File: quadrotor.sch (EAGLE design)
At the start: 10 parts, among them X1 16MHZ

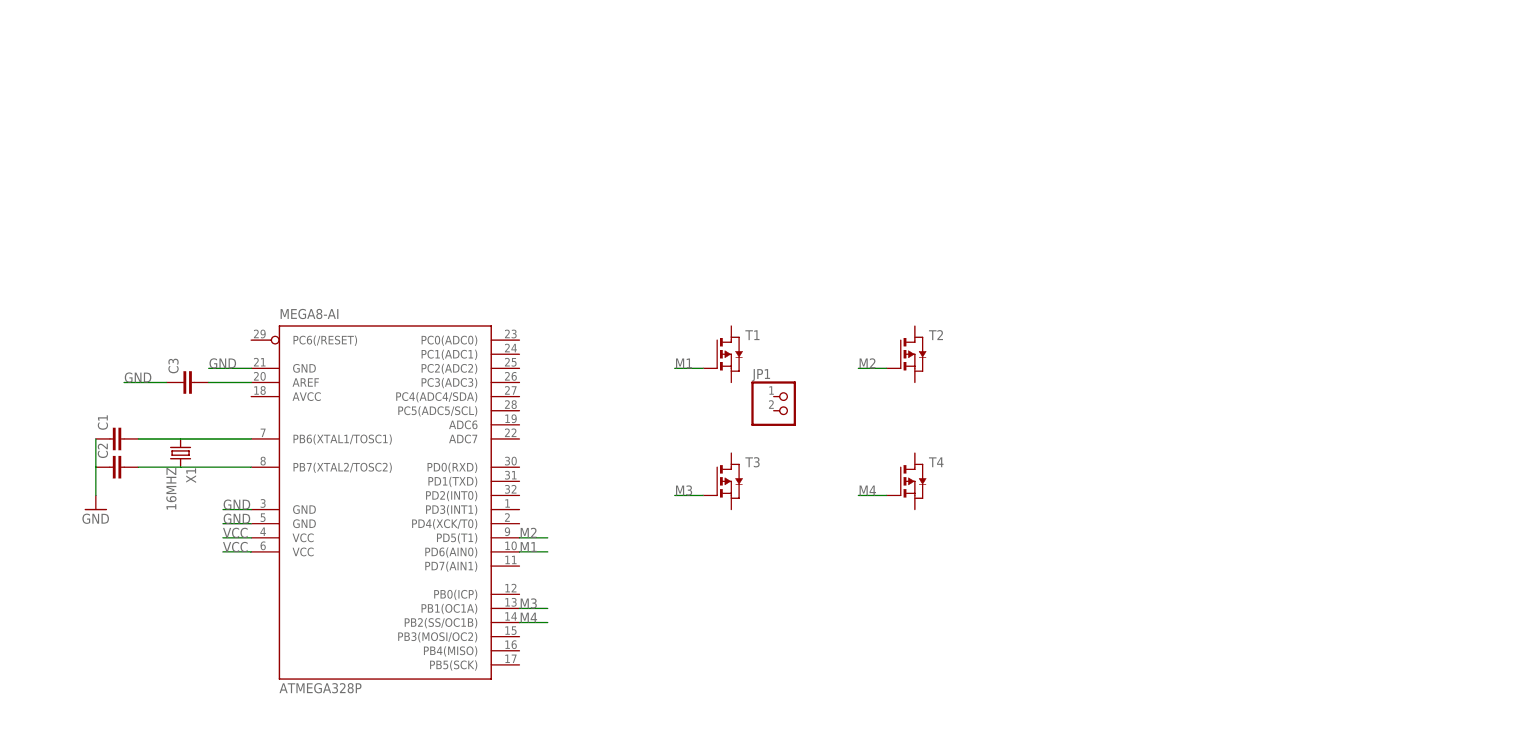
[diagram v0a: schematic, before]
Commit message: done bluetooth protocal
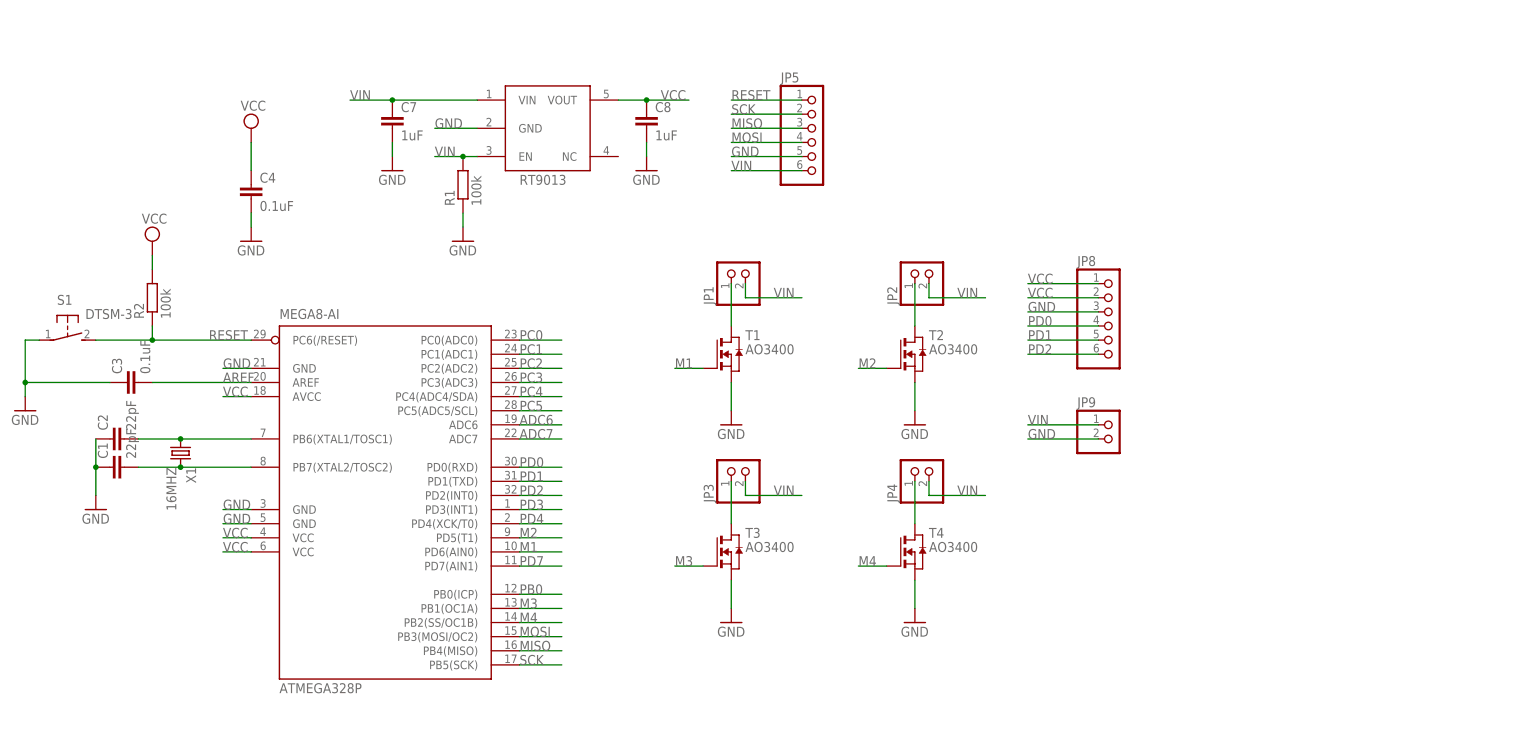
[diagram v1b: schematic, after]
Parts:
- added C4: 0.1uF, eagle-ltspice:CC0603
- added C7, C8: 1uF, eagle-ltspice:CC0603
- added JP2, JP3, JP4: (no value), pinhead:PINHD-1X2
- added JP5: (no value), pinhead:PINHD-1X6/90
- added JP8: (no value), pinhead:PINHD-1X6
- added JP9: (no value), pinhead:PINHD-1X2/90
- added R1, R2: 100k, eagle-ltspice:RR0603
- added S1: DTSM-3, switch-tact:DTSM-3
- added U$1: RT9013, quadrotor:RT9013
- C1, C2: value (none) -> 22pF
- C3: value (none) -> 0.1uF
- T1, T2, T3, T4: value (none) -> AO3400; device zetex:PMOSSOT23 -> zetex:NMOSSOT23
- X1: device IQD-Frequency-Products:CRYSTALS-NOGND-HC49 -> IQD-Frequency-Products:CRYSTALS-NOGND-12SMX-A
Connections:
- net N$3 renamed AREF
- new net ADC6: ATMEGA328P.ADC6
- new net ADC7: ATMEGA328P.ADC7
- new net MISO: ATMEGA328P.PB4(MISO), JP5.3
- new net MOSI: ATMEGA328P.PB3(MOSI/OC2), JP5.4
- new net N$10: JP3.1, T3.D
- new net N$4: JP1.1, T1.D
- new net N$6: JP2.1, T2.D
- new net N$9: JP4.1, T4.D
- new net PB0: ATMEGA328P.PB0(ICP)
- new net PC0: ATMEGA328P.PC0(ADC0)
- new net PC1: ATMEGA328P.PC1(ADC1)
- new net PC2: ATMEGA328P.PC2(ADC2)
- new net PC3: ATMEGA328P.PC3(ADC3)
- new net PC4: ATMEGA328P.PC4(ADC4/SDA)
- new net PC5: ATMEGA328P.PC5(ADC5/SCL)
- new net PD0: ATMEGA328P.PD0(RXD), JP8.4
- new net PD1: ATMEGA328P.PD1(TXD), JP8.5
- new net PD2: ATMEGA328P.PD2(INT0), JP8.6
- new net PD3: ATMEGA328P.PD3(INT1)
- new net PD4: ATMEGA328P.PD4(XCK/T0)
- new net PD7: ATMEGA328P.PD7(AIN1)
- new net RESET: ATMEGA328P.PC6(/RESET), JP5.1, R2.1, S1.2
- new net SCK: ATMEGA328P.PB5(SCK), JP5.2
- new net VIN: C7.1, JP1.2, JP2.2, JP3.2, JP4.2, JP5.6, JP9.1, R1.2, U$1.EN, U$1.VIN
- net GND: now also C4.2, C7.2, C8.2, JP5.5, JP8.3, JP9.2, R1.1, S1.1, T1.S, T2.S, T3.S, T4.S, U$1.GND
- net N$1: now also C2.2; no longer C1.2
- net N$2: now also C1.2; no longer C2.2
- net VCC: now also ATMEGA328P.AVCC, C4.1, C8.1, JP8.1, JP8.2, R2.2, U$1.VOUT
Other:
- moved on the sheet: C1, C2, C3, JP1, T3, T4

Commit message: mostly done layout and is routing now
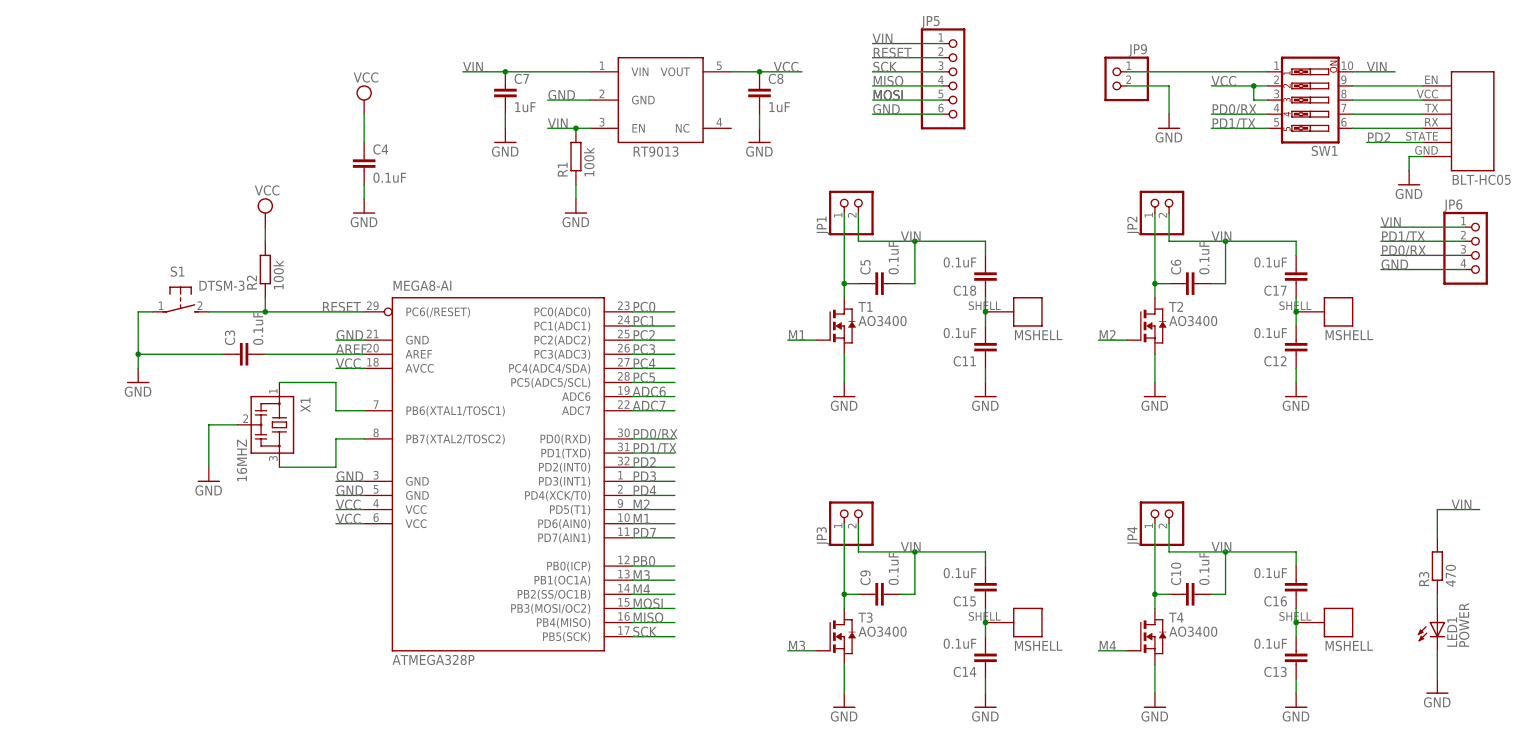
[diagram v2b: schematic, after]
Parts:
- removed C1, C2: 22pF, eagle-ltspice:CC0603
- removed JP8: (no value), pinhead:PINHD-1X6
- added C10, C11, C12, C13, C14, C15, C16, C17, C18, C5, C6, C9: 0.1uF, eagle-ltspice:CC0603
- added JP6: (no value), pinhead:PINHD-1X4
- added LED1: POWER, eagle-ltspice:LED_ESML0603
- added R3: 470, eagle-ltspice:RR0603
- added SW1: (no value), special:SW_DIP-5
- added U$2: BLT-HC05, quadrotor:BLT-HC05
- added U$3, U$4, U$5, U$6: 720-MSHELL, quadrotor:720-MSHELL
- JP5: device pinhead:PINHD-1X6/90 -> pinhead:PINHD-1X6
- JP9: device pinhead:PINHD-1X2/90 -> pinhead:PINHD-1X2
- X1: device IQD-Frequency-Products:CRYSTALS-NOGND-12SMX-A -> murata-filter:CSTCR6M00G53Z
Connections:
- removed net PD0: ATMEGA328P.PD0(RXD), JP8.4
- removed net PD1: ATMEGA328P.PD1(TXD), JP8.5
- new net N$11: SW1.8, U$2.VCC
- new net N$12: SW1.7, U$2.TX
- new net N$13: SW1.6, U$2.RX
- new net N$14: JP9.1, SW1.1
- new net N$15: C12.2, C17.1, U$4.SHELL
- new net N$16: C13.2, C16.1, U$6.SHELL
- new net N$3: C14.2, C15.1, U$5.SHELL
- new net N$5: C11.2, C18.1, U$3.SHELL
- new net N$7: SW1.9, U$2.EN
- new net N$8: LED1.A, R3.1
- new net PD0/RX: ATMEGA328P.PD0(RXD), JP6.3, SW1.4
- new net PD1/TX: ATMEGA328P.PD1(TXD), JP6.2, SW1.5
- net GND: now also C11.1, C12.1, C13.1, C14.1, JP5.6, JP6.4, LED1.C, U$2.GND, X1.2; no longer C1.1, C2.1, JP5.5, JP8.3
- net MISO: now also JP5.4; no longer JP5.3
- net MOSI: now also JP5.5; no longer JP5.4
- net N$1: no longer C2.2
- net N$10: now also C9.1
- net N$2: now also X1.3; no longer C1.2, X1.2
- net N$4: now also C5.1
- net N$6: now also C6.1
- net N$9: now also C10.1
- net PD2: now also U$2.STATE; no longer JP8.6
- net RESET: now also JP5.2; no longer JP5.1
- net SCK: now also JP5.3; no longer JP5.2
- net VCC: now also SW1.2, SW1.3; no longer JP8.1, JP8.2
- net VIN: now also C10.2, C15.2, C16.2, C17.2, C18.2, C5.2, C6.2, C9.2, JP5.1, JP6.1, R3.2, SW1.10; no longer JP5.6, JP9.1
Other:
- moved on the sheet: ATMEGA328P, C3, C4, C7, C8, JP1, JP2, JP3, JP4, JP5, JP9, R1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
